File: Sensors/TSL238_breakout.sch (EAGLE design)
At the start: 4 parts

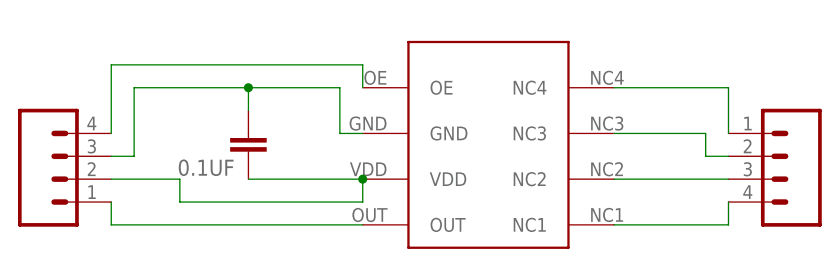
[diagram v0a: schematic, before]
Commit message: updated tsl238
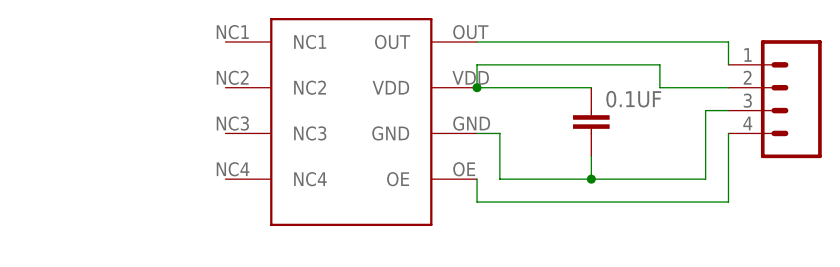
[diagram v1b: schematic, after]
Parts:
- removed J2: (no value), SparkFun-Connectors:M04PTH
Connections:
- net N$5 renamed OE
- net N$6 renamed VCC
- net N$8 renamed OUT
- net N$9 renamed GND
- removed net N$1: J2.1, U$1.NC4
- removed net N$2: J2.2, U$1.NC3
- removed net N$3: J2.3, U$1.NC2
- removed net N$4: J2.4, U$1.NC1
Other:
- moved on the sheet: 0.1UF
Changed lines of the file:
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@@
 <?xml version="1.0" encoding="utf-8"?>
 <!DOCTYPE eagle SYSTEM "eagle.dtd">
-<eagle version="7.3.0">
+<eagle version="7.7.0">
 <drawing>
 <settings>
@@
 <part name="0.1UF" library="SparkFun-Capacitors" deviceset="CAP" device="0603-CAP"/>
 <part name="J1" library="SparkFun-Connectors" deviceset="M04" device="PTH"/>
-<part name="J2" library="SparkFun-Connectors" deviceset="M04" device="PTH"/>
 </parts>
 <sheets>
@@
 </plain>
 <instances>
-<instance part="U$1" gate="G$1" x="55.88" y="12.7" rot="R90"/>
-<instance part="0.1UF" gate="G$1" x="27.94" y="15.24" rot="R180"/>
-<instance part="J1" gate="G$1" x="7.62" y="10.16" smashed="yes">
-<attribute name="VALUE" x="2.54" y="2.54" size="1.778" layer="96"/>
-</instance>
-<instance part="J2" gate="G$1" x="86.36" y="12.7" smashed="yes" rot="R180">
-<attribute name="VALUE" x="91.44" y="20.32" size="1.778" layer="96" rot="R180"/>
+<instance part="U$1" gate="G$1" x="38.1" y="17.78" rot="R270"/>
+<instance part="0.1UF" gate="G$1" x="66.04" y="15.24"/>
+<instance part="J1" gate="G$1" x="86.36" y="20.32" smashed="yes" rot="R180">
+<attribute name="VALUE" x="91.44" y="27.94" size="1.778" layer="96" rot="R180"/>
 </instance>
 </instances>
@@
 </busses>
 <nets>
-<net name="N$1" class="0">
-<segment>
-<pinref part="U$1" gate="G$1" pin="NC4"/>
-<pinref part="J2" gate="G$1" pin="1"/>
-<wire x1="68.58" y1="20.32" x2="81.28" y2="20.32" width="0.1524" layer="91"/>
-<wire x1="81.28" y1="20.32" x2="81.28" y2="15.24" width="0.1524" layer="91"/>
-</segment>
-</net>
-<net name="N$2" class="0">
-<segment>
-<pinref part="U$1" gate="G$1" pin="NC3"/>
-<wire x1="68.58" y1="15.24" x2="78.74" y2="15.24" width="0.1524" layer="91"/>
-<wire x1="78.74" y1="15.24" x2="78.74" y2="12.7" width="0.1524" layer="91"/>
-<pinref part="J2" gate="G$1" pin="2"/>
-<wire x1="78.74" y1="12.7" x2="81.28" y2="12.7" width="0.1524" layer="91"/>
-</segment>
-</net>
-<net name="N$3" class="0">
-<segment>
-<pinref part="U$1" gate="G$1" pin="NC2"/>
-<pinref part="J2" gate="G$1" pin="3"/>
-<wire x1="68.58" y1="10.16" x2="81.28" y2="10.16" width="0.1524" layer="91"/>
-</segment>
-</net>
-<net name="N$4" class="0">
-<segment>
-<pinref part="U$1" gate="G$1" pin="NC1"/>
-<pinref part="J2" gate="G$1" pin="4"/>
-<wire x1="68.58" y1="5.08" x2="81.28" y2="5.08" width="0.1524" layer="91"/>
-<wire x1="81.28" y1="5.08" x2="81.28" y2="7.62" width="0.1524" layer="91"/>
-</segment>
-</net>
-<net name="N$5" class="0">
+<net name="OE" class="0">
 <segment>
 <pinref part="U$1" gate="G$1" pin="OE"/>
-<wire x1="40.64" y1="20.32" x2="40.64" y2="22.86" width="0.1524" layer="91"/>
+<wire x1="53.34" y1="10.16" x2="53.34" y2="7.62" width="0.1524" layer="91"/>
 <pinref part="J1" gate="G$1" pin="4"/>
-<wire x1="40.64" y1="22.86" x2="12.7" y2="22.86" width="0.1524" layer="91"/>
-<wire x1="12.7" y1="22.86" x2="12.7" y2="15.24" width="0.1524" layer="91"/>
-</segment>
-</net>
-<net name="N$8" class="0">
+<wire x1="53.34" y1="7.62" x2="81.28" y2="7.62" width="0.1524" layer="91"/>
+<wire x1="81.28" y1="7.62" x2="81.28" y2="15.24" width="0.1524" layer="91"/>
+</segment>
+</net>
+<net name="OUT" class="0">
 <segment>
 <pinref part="U$1" gate="G$1" pin="OUT"/>
 <pinref part="J1" gate="G$1" pin="1"/>
-<wire x1="40.64" y1="5.08" x2="12.7" y2="5.08" width="0.1524" layer="91"/>
-<wire x1="12.7" y1="5.08" x2="12.7" y2="7.62" width="0.1524" layer="91"/>
-</segment>
-</net>
-<net name="N$9" class="0">
-<segment>
-<wire x1="15.24" y1="20.32" x2="15.24" y2="12.7" width="0.1524" layer="91"/>
+<wire x1="53.34" y1="25.4" x2="81.28" y2="25.4" width="0.1524" layer="91"/>
+<wire x1="81.28" y1="25.4" x2="81.28" y2="22.86" width="0.1524" layer="91"/>
+</segment>
+</net>
+<net name="GND" class="0">
+<segment>
+<wire x1="78.74" y1="10.16" x2="78.74" y2="17.78" width="0.1524" layer="91"/>
 <pinref part="J1" gate="G$1" pin="3"/>
-<wire x1="15.24" y1="12.7" x2="12.7" y2="12.7" width="0.1524" layer="91"/>
-<wire x1="15.24" y1="20.32" x2="27.94" y2="20.32" width="0.1524" layer="91"/>
-<wire x1="27.94" y1="20.32" x2="38.1" y2="20.32" width="0.1524" layer="91"/>
-<wire x1="38.1" y1="20.32" x2="38.1" y2="15.24" width="0.1524" layer="91"/>
+<wire x1="78.74" y1="17.78" x2="81.28" y2="17.78" width="0.1524" layer="91"/>
+<wire x1="78.74" y1="10.16" x2="66.04" y2="10.16" width="0.1524" layer="91"/>
+<wire x1="66.04" y1="10.16" x2="55.88" y2="10.16" width="0.1524" layer="91"/>
+<wire x1="55.88" y1="10.16" x2="55.88" y2="15.24" width="0.1524" layer="91"/>
 <pinref part="U$1" gate="G$1" pin="GND"/>
-<wire x1="38.1" y1="15.24" x2="40.64" y2="15.24" width="0.1524" layer="91"/>
+<wire x1="55.88" y1="15.24" x2="53.34" y2="15.24" width="0.1524" layer="91"/>
 <pinref part="0.1UF" gate="G$1" pin="2"/>
-<wire x1="27.94" y1="17.78" x2="27.94" y2="20.32" width="0.1524" layer="91"/>
-<junction x="27.94" y="20.32"/>
-</segment>
-</net>
-<net name="N$6" class="0">
+<wire x1="66.04" y1="12.7" x2="66.04" y2="10.16" width="0.1524" layer="91"/>
+<junction x="66.04" y="10.16"/>
+</segment>
+</net>
+<net name="VCC" class="0">
 <segment>
 <pinref part="J1" gate="G$1" pin="2"/>
-<wire x1="20.32" y1="10.16" x2="12.7" y2="10.16" width="0.1524" layer="91"/>
-<wire x1="20.32" y1="10.16" x2="20.32" y2="7.62" width="0.1524" layer="91"/>
+<wire x1="73.66" y1="20.32" x2="81.28" y2="20.32" width="0.1524" layer="91"/>
+<wire x1="73.66" y1="20.32" x2="73.66" y2="22.86" width="0.1524" layer="91"/>
 <pinref part="0.1UF" gate="G$1" pin="1"/>
 <pinref part="U$1" gate="G$1" pin="VDD"/>
-<wire x1="40.64" y1="10.16" x2="27.94" y2="10.16" width="0.1524" layer="91"/>
-<wire x1="20.32" y1="7.62" x2="40.64" y2="7.62" width="0.1524" layer="91"/>
-<wire x1="40.64" y1="7.62" x2="40.64" y2="10.16" width="0.1524" layer="91"/>
-<junction x="40.64" y="10.16"/>
-</segment>
-</net>
+<wire x1="53.34" y1="20.32" x2="66.04" y2="20.32" width="0.1524" layer="91"/>
+<wire x1="73.66" y1="22.86" x2="53.34" y2="22.86" width="0.1524" layer="91"/>
+<wire x1="53.34" y1="22.86" x2="53.34" y2="20.32" width="0.1524" layer="91"/>
+<junction x="53.34" y="20.32"/>
+</segment>
+</net>
